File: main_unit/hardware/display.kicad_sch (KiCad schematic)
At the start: 30 parts, among them J1 62684-402100ALF, Q1 2N7002BK,215, U4 MAX25512ATG/V+T

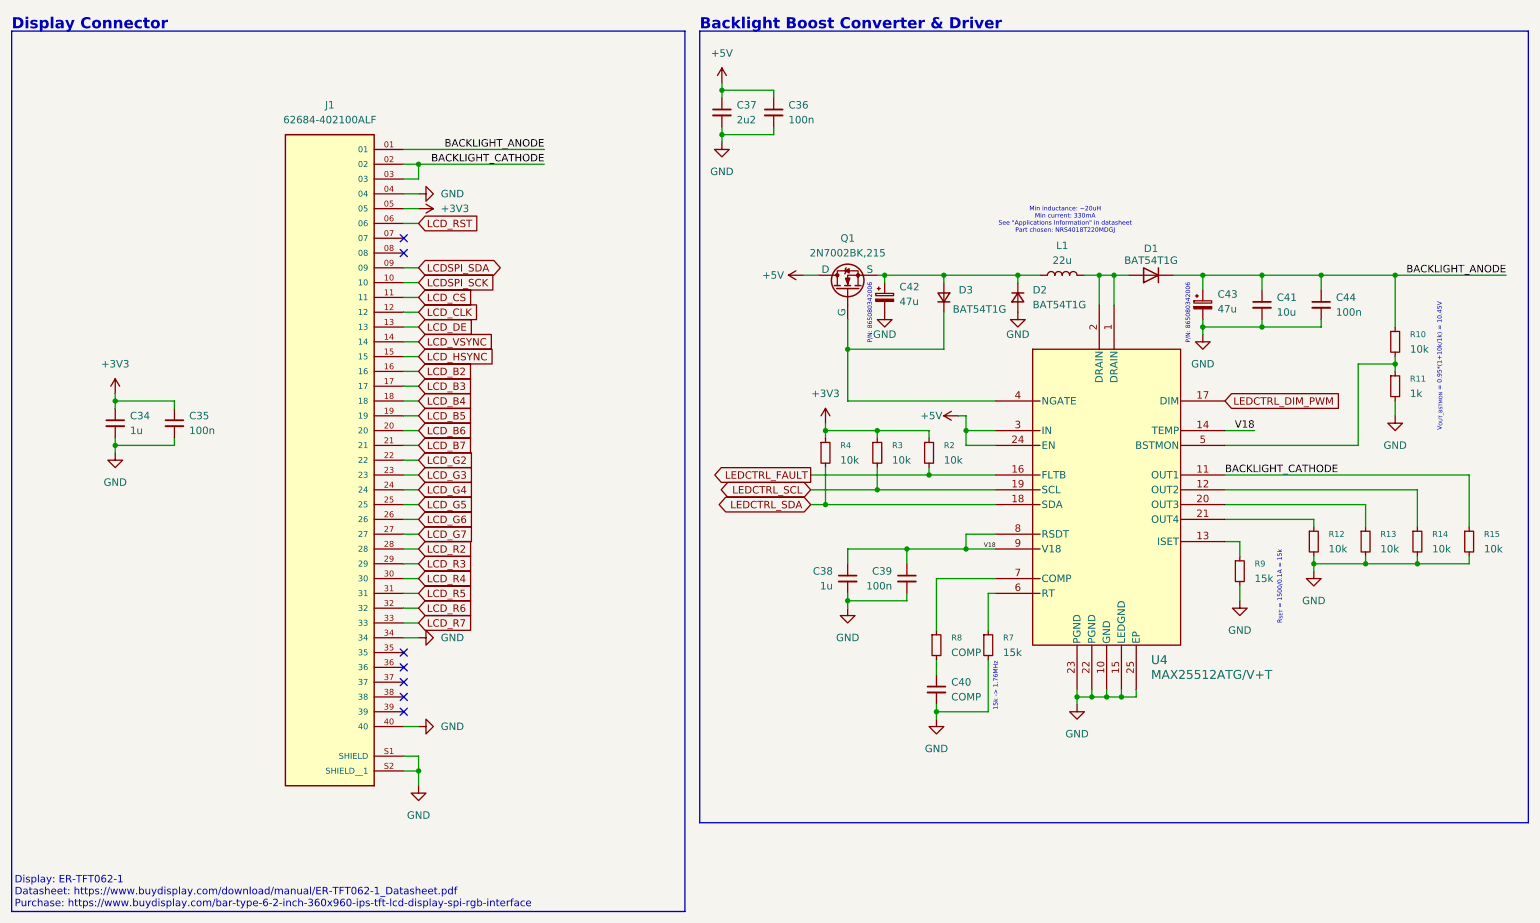
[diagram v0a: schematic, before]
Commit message: main_unit/hardware: Fill in compensation circuit values
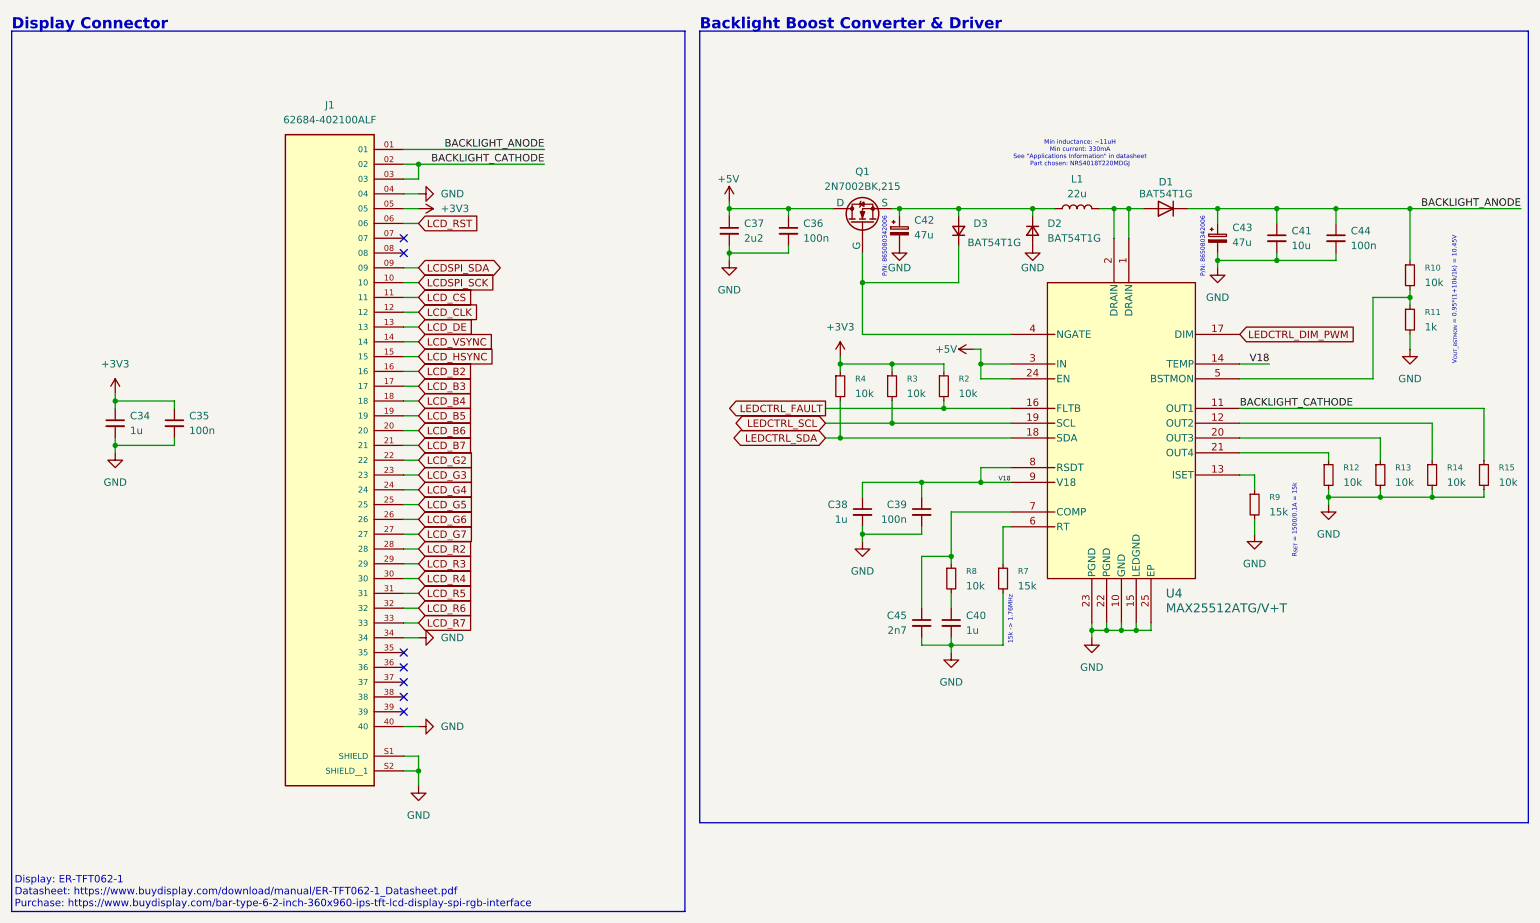
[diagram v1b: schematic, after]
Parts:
- added C45: 2n7, Capacitor_SMD:C_0201_0603Metric, symbol Device:C_Small
- C40: value COMP -> 1u; footprint Capacitor_SMD:C_0603_1608Metric -> Capacitor_SMD:C_0805_2012Metric
- R8: value COMP -> 10k
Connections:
- net GND: now also C45.2
- net at R8.1, U4.7 (COMP): now also C45.1
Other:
- note added: "Min inductance: ~11uH Min current: 330mA See "Applications Information" in datasheet Part chosen: NRS4018T220MDGJ"
- note removed: "Min inductance: ~20uH Min current: 330mA See "Applications Information" in datasheet Part chosen: NRS4018T220MDGJ"
- moved on the sheet: C36, C37, C38, C39, C40, C41, C42, C43, C44, D1, D2, D3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
